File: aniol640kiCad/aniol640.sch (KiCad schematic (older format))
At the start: 38 parts, among them J1 RST, J2 PWR, U12 74LS74, U2 74LS14, U4 74LS32, U5 74LS08, X1 ACO-1.8432MHz

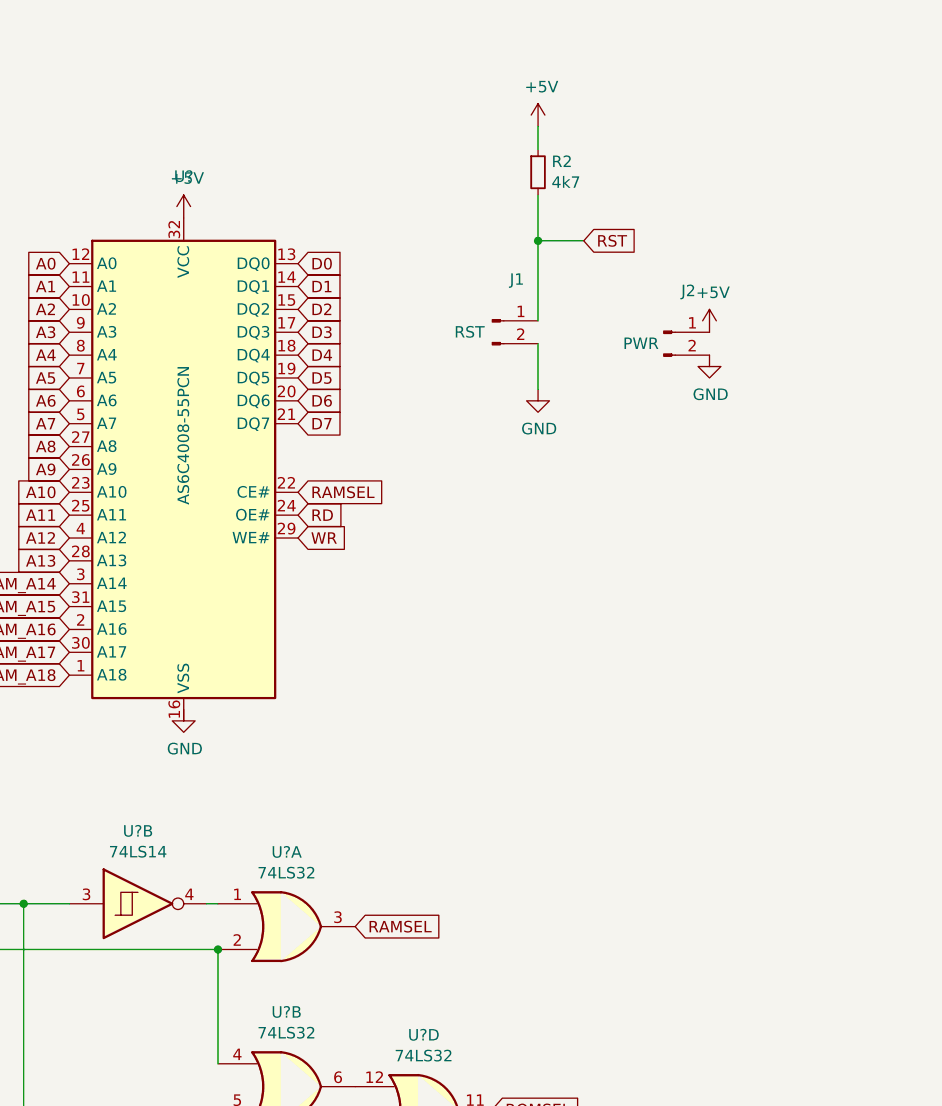
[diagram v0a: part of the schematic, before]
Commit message: developing the skbd module
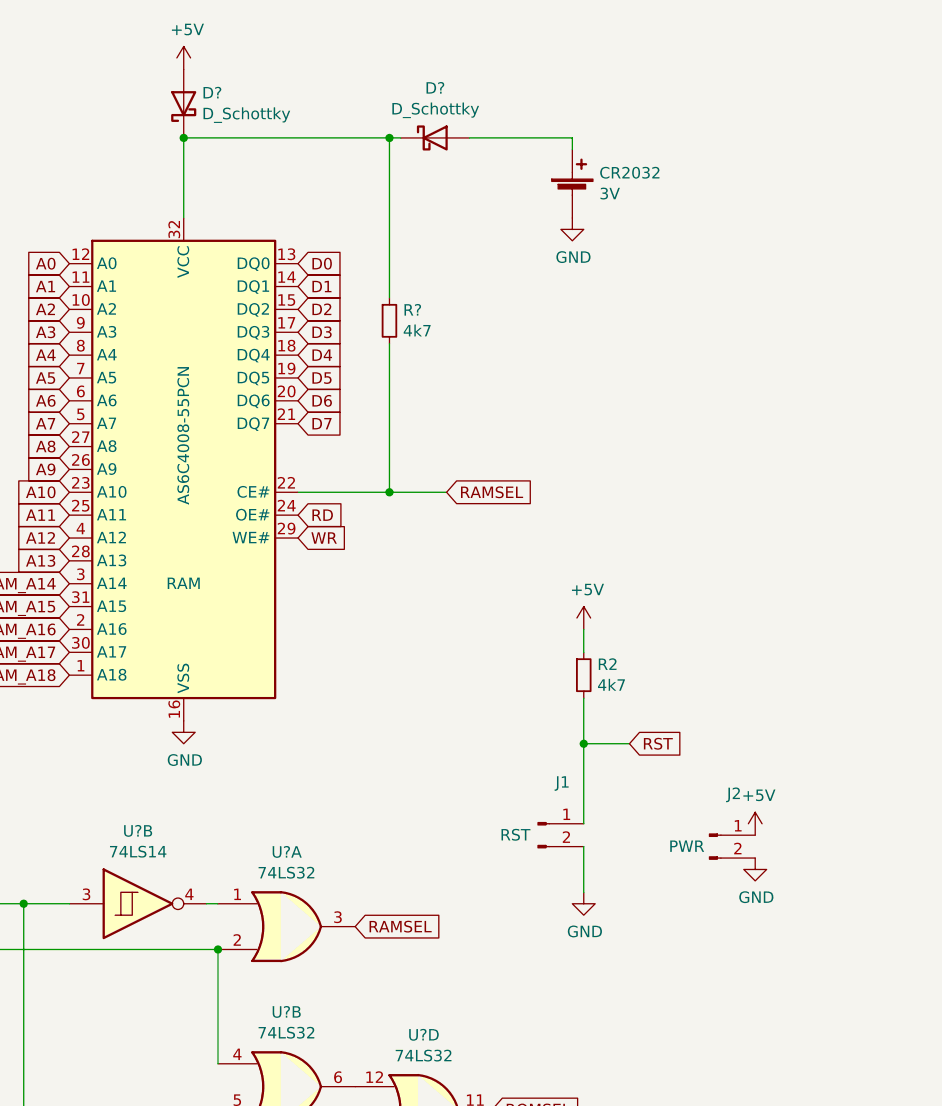
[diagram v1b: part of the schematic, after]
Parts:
- added CR2032: 3V, symbol Device:Battery_Cell
- added D? (x2): D_Schottky, symbol Device:D_Schottky
- added R?: 4k7, symbol Device:R_Small
- gave numbers to parts that had none: 1
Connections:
- net +5V: now also D?.2 (A); no longer RAM.32 (VCC)
- net GND: now also RAM.16 (VSS), CR2032.2 (-)
- net RAMSEL: now also R?.2
- new net: D?.1 (K), D?.1 (K), R?.1, RAM.32 (VCC)
- new net: CR2032.1 (+), D?.2 (A)
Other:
- moved on the sheet: J1, J2, R2
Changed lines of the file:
@@
 L power:GND #PWR02
 U 1 1 61D165C5
-P 10000 2500
-F 0 "#PWR02" H 10000 2250 50  0001 C CNN
-F 1 "GND" H 10005 2327 50  0000 C CNN
-F 2 "" H 10000 2500 50  0001 C CNN
-F 3 "" H 10000 2500 50  0001 C CNN
-	1    10000 2500
+P 10200 4700
+F 0 "#PWR02" H 10200 4450 50  0001 C CNN
+F 1 "GND" H 10205 4527 50  0000 C CNN
+F 2 "" H 10200 4700 50  0001 C CNN
+F 3 "" H 10200 4700 50  0001 C CNN
+	1    10200 4700
 	1    0    0    -1
 $EndComp
@@
 L power:+5V #PWR01
 U 1 1 61D16900
-P 10000 1350
-F 0 "#PWR01" H 10000 1200 50  0001 C CNN
-F 1 "+5V" H 10015 1523 50  0000 C CNN
-F 2 "" H 10000 1350 50  0001 C CNN
-F 3 "" H 10000 1350 50  0001 C CNN
-	1    10000 1350
+P 10200 3550
+F 0 "#PWR01" H 10200 3400 50  0001 C CNN
+F 1 "+5V" H 10215 3723 50  0000 C CNN
+F 2 "" H 10200 3550 50  0001 C CNN
+F 3 "" H 10200 3550 50  0001 C CNN
+	1    10200 3550
 	1    0    0    -1
 $EndComp
@@
 L Device:R_Small R2
 U 1 1 61D1747F
-P 10000 1550
-F 0 "R2" H 10059 1596 50  0000 L CNN
-F 1 "4k7" H 10059 1505 50  0000 L CNN
-F 2 "Resistor_THT:R_Axial_DIN0207_L6.3mm_D2.5mm_P7.62mm_Horizontal" H 10000 1550 50  0001 C CNN
-F 3 "~" H 10000 1550 50  0001 C CNN
-	1    10000 1550
-	1    0    0    -1
-$EndComp
-Wire Wire Line
-	10000 1350 10000 1450
-Wire Wire Line
-	10000 1650 10000 1850
-Text GLabel 10200 1850 2    50   Input ~ 0
+P 10200 3750
+F 0 "R2" H 10259 3796 50  0000 L CNN
+F 1 "4k7" H 10259 3705 50  0000 L CNN
+F 2 "Resistor_THT:R_Axial_DIN0207_L6.3mm_D2.5mm_P7.62mm_Horizontal" H 10200 3750 50  0001 C CNN
+F 3 "~" H 10200 3750 50  0001 C CNN
+	1    10200 3750
+	1    0    0    -1
+$EndComp
+Wire Wire Line
+	10200 3550 10200 3650
+Wire Wire Line
+	10200 3850 10200 4050
+Text GLabel 10400 4050 2    50   Input ~ 0
 RST
 Wire Wire Line
-	10200 1850 10000 1850
-Connection ~ 10000 1850
+	10400 4050 10200 4050
+Connection ~ 10200 4050
 $Comp
 L 74xx:74LS08 U5
@@
 L Connector:Conn_01x02_Male J2
 U 1 1 61D552DF
-P 10550 2250
-F 0 "J2" H 10658 2431 50  0000 C CNN
-F 1 "PWR" H 10450 2200 50  0000 C CNN
-F 2 "Connector_PinHeader_2.54mm:PinHeader_1x02_P2.54mm_Vertical" H 10550 2250 50  0001 C CNN
-F 3 "~" H 10550 2250 50  0001 C CNN
-	1    10550 2250
+P 10750 4450
+F 0 "J2" H 10858 4631 50  0000 C CNN
+F 1 "PWR" H 10650 4400 50  0000 C CNN
+F 2 "Connector_PinHeader_2.54mm:PinHeader_1x02_P2.54mm_Vertical" H 10750 4450 50  0001 C CNN
+F 3 "~" H 10750 4450 50  0001 C CNN
+	1    10750 4450
 	1    0    0    -1
 $EndComp
@@
 L power:GND #PWR06
 U 1 1 61D56634
-P 10750 2350
-F 0 "#PWR06" H 10750 2100 50  0001 C CNN
-F 1 "GND" H 10755 2177 50  0000 C CNN
-F 2 "" H 10750 2350 50  0001 C CNN
-F 3 "" H 10750 2350 50  0001 C CNN
-	1    10750 2350
+P 10950 4550
+F 0 "#PWR06" H 10950 4300 50  0001 C CNN
+F 1 "GND" H 10955 4377 50  0000 C CNN
+F 2 "" H 10950 4550 50  0001 C CNN
+F 3 "" H 10950 4550 50  0001 C CNN
+	1    10950 4550
 	1    0    0    -1
 $EndComp
@@
 L power:+5V #PWR05
 U 1 1 61D56F4A
-P 10750 2250
-F 0 "#PWR05" H 10750 2100 50  0001 C CNN
-F 1 "+5V" H 10765 2423 50  0000 C CNN
-F 2 "" H 10750 2250 50  0001 C CNN
-F 3 "" H 10750 2250 50  0001 C CNN
-	1    10750 2250
+P 10950 4450
+F 0 "#PWR05" H 10950 4300 50  0001 C CNN
+F 1 "+5V" H 10965 4623 50  0000 C CNN
+F 2 "" H 10950 4450 50  0001 C CNN
+F 3 "" H 10950 4450 50  0001 C CNN
+	1    10950 4450
 	1    0    0    -1
 $EndComp
@@
 L Connector:Conn_01x02_Male J1
 U 1 1 61D57B45
-P 9800 2200
-F 0 "J1" H 9908 2381 50  0000 C CNN
-F 1 "RST" H 9700 2150 50  0000 C CNN
-F 2 "Connector_PinHeader_2.54mm:PinHeader_1x02_P2.54mm_Vertical" H 9800 2200 50  0001 C CNN
-F 3 "~" H 9800 2200 50  0001 C CNN
-	1    9800 2200
-	1    0    0    -1
-$EndComp
-Wire Wire Line
-	10000 1850 10000 2200
-Wire Wire Line
-	10000 2300 10000 2500
+P 10000 4400
+F 0 "J1" H 10108 4581 50  0000 C CNN
+F 1 "RST" H 9900 4350 50  0000 C CNN
+F 2 "Connector_PinHeader_2.54mm:PinHeader_1x02_P2.54mm_Vertical" H 10000 4400 50  0001 C CNN
+F 3 "~" H 10000 4400 50  0001 C CNN
+	1    10000 4400
+	1    0    0    -1
+$EndComp
+Wire Wire Line
+	10200 4050 10200 4400
+Wire Wire Line
+	10200 4500 10200 4700
 Wire Wire Line
 	2150 2200 2150 2800
@@
 L power:+5V #PWR?
 U 1 1 62297CAA
-P 8450 1750
-F 0 "#PWR?" H 8450 1600 50  0001 C CNN
-F 1 "+5V" H 8465 1923 50  0000 C CNN
-F 2 "" H 8450 1750 50  0001 C CNN
-F 3 "" H 8450 1750 50  0001 C CNN
-	1    8450 1750
+P 8450 1100
+F 0 "#PWR?" H 8450 950 50  0001 C CNN
+F 1 "+5V" H 8465 1273 50  0000 C CNN
+F 2 "" H 8450 1100 50  0001 C CNN
+F 3 "" H 8450 1100 50  0001 C CNN
+	1    8450 1100
 	1    0    0    -1
 $EndComp
@@
 L power:GND #PWR?
 U 1 1 622986B6
-P 8450 3900
-F 0 "#PWR?" H 8450 3650 50  0001 C CNN
-F 1 "GND" H 8455 3727 50  0000 C CNN
-F 2 "" H 8450 3900 50  0001 C CNN
-F 3 "" H 8450 3900 50  0001 C CNN
-	1    8450 3900
+P 8450 3950
+F 0 "#PWR?" H 8450 3700 50  0001 C CNN
+F 1 "GND" H 8455 3777 50  0000 C CNN
+F 2 "" H 8450 3950 50  0001 C CNN
+F 3 "" H 8450 3950 50  0001 C CNN
+	1    8450 3950
 	1    0    0    -1
 $EndComp
@@
 Text GLabel 6100 3550 0    50   Input ~ 0
 ROMSEL
-Text GLabel 8950 2950 2    50   Input ~ 0
+Text GLabel 9600 2950 2    50   Input ~ 0
 RAMSEL
 Text GLabel 7950 1950 0    50   Input ~ 0
@@
 ROMSEL
 $Comp
-L Memory_RAM:AS6C4008-55PCN U?
+L Memory_RAM:AS6C4008-55PCN RAM
 U 1 1 6248C2B7
 P 8450 2850
-F 0 "U?" H 8450 4131 50  0000 C CNN
+F 0 "RAM" H 8450 2350 50  0000 C CNN
 F 1 "AS6C4008-55PCN" V 8450 3000 50  0000 C CNN
 F 2 "Package_DIP:DIP-32_W15.24mm" H 8450 2950 50  0001 C CNN
@@
 Wire Wire Line
 	4300 6050 4650 6050
+$Comp
+L Device:D_Schottky D?
+U 1 1 625B1E53
+P 8450 1250
+F 0 "D?" V 8496 1170 50  0000 R CNN
+F 1 "D_Schottky" V 8405 1170 50  0000 R CNN
+F 2 "" H 8450 1250 50  0001 C CNN
+F 3 "~" H 8450 1250 50  0001 C CNN
+	1    8450 1250
+	0    -1   -1   0
+$EndComp
+$Comp
+L Device:D_Schottky D?
+U 1 1 625B23EB
+P 9550 1400
+F 0 "D?" H 9550 1617 50  0000 C CNN
+F 1 "D_Schottky" H 9550 1526 50  0000 C CNN
+F 2 "" H 9550 1400 50  0001 C CNN
+F 3 "~" H 9550 1400 50  0001 C CNN
+	1    9550 1400
+	1    0    0    -1
+$EndComp
+Wire Wire Line
+	8450 1400 8450 1750
+Connection ~ 8450 1400
+Wire Wire Line
+	8450 1400 9350 1400
+$Comp
+L Device:R_Small R?
+U 1 1 625D62BC
+P 9350 2200
+F 0 "R?" H 9409 2246 50  0000 L CNN
+F 1 "4k7" H 9409 2155 50  0000 L CNN
+F 2 "" H 9350 2200 50  0001 C CNN
+F 3 "~" H 9350 2200 50  0001 C CNN
+	1    9350 2200
+	1    0    0    -1
+$EndComp
+Wire Wire Line
+	9350 1400 9350 2100
+Connection ~ 9350 1400
+Wire Wire Line
+	9350 1400 9400 1400
+Wire Wire Line
+	9350 2300 9350 2950
+Wire Wire Line
+	9350 2950 8950 2950
+Wire Wire Line
+	9350 2950 9600 2950
+Connection ~ 9350 2950
+$Comp
+L Device:Battery_Cell CR2032
+U 1 1 625E844B
+P 10150 1650
+F 0 "CR2032" H 10268 1746 50  0000 L CNN
+F 1 "3V" H 10268 1655 50  0000 L CNN
+F 2 "" V 10150 1710 50  0001 C CNN
+F 3 "~" V 10150 1710 50  0001 C CNN
+	1    10150 1650
+	1    0    0    -1
+$EndComp
+Wire Wire Line
+	10150 1450 10150 1400
+Wire Wire Line
+	10150 1400 9700 1400
+$Comp
+L power:GND #PWR?
+U 1 1 625F0565
+P 10150 1750
+F 0 "#PWR?" H 10150 1500 50  0001 C CNN
+F 1 "GND" H 10155 1577 50  0000 C CNN
+F 2 "" H 10150 1750 50  0001 C CNN
+F 3 "" H 10150 1750 50  0001 C CNN
+	1    10150 1750
+	1    0    0    -1
+$EndComp
 $EndSCHEMATC
